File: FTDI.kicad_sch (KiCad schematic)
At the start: 14 parts, among them U6 FT2232HL-TRAY, Y2 12Mhz 20ppm

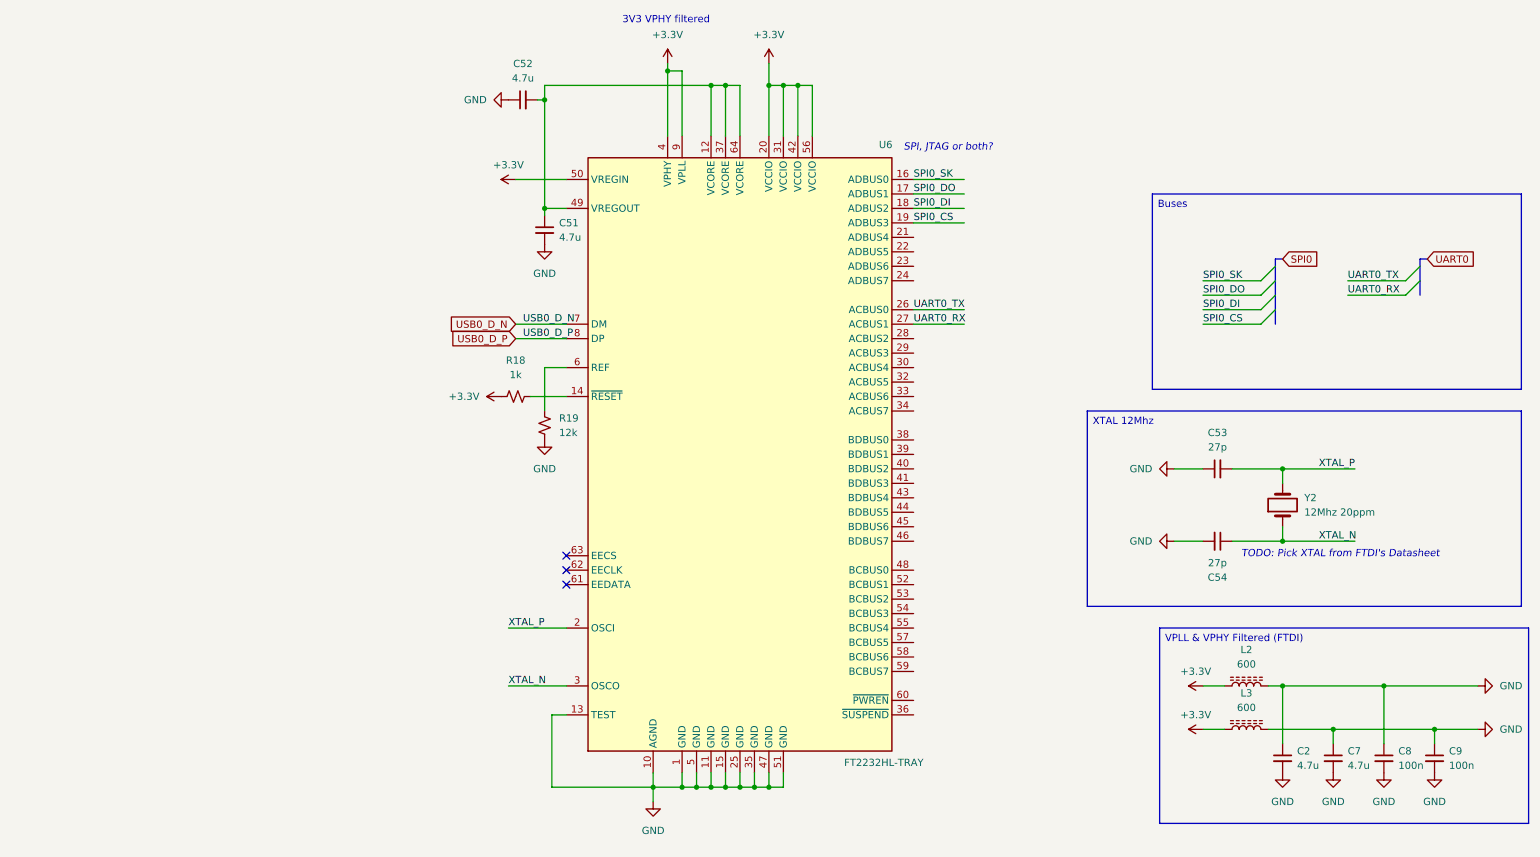
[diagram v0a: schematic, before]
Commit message: Alot of stuff
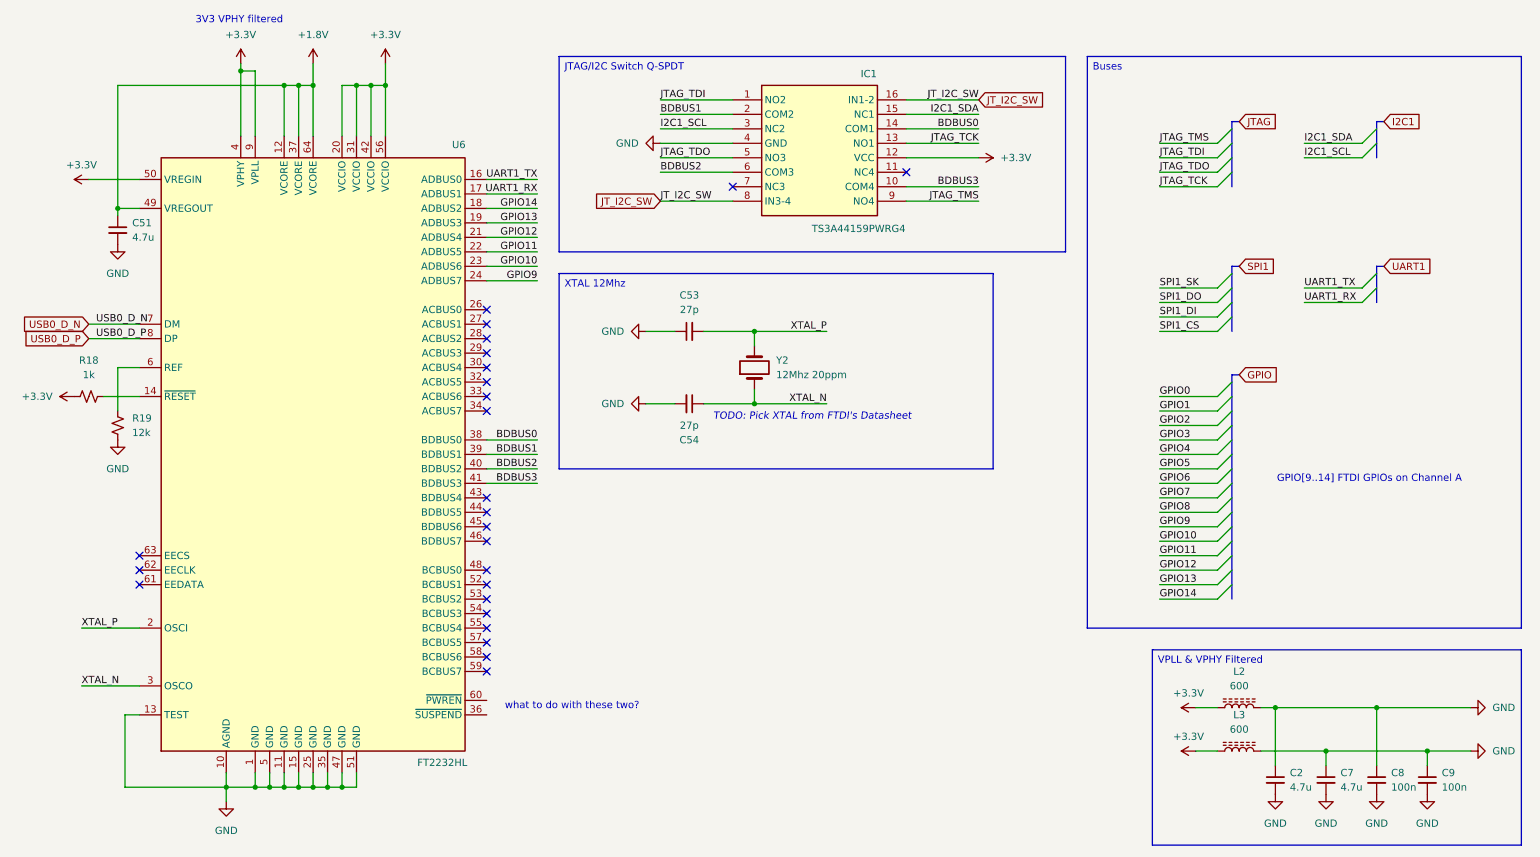
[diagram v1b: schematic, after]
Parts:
- removed C52: 4.7u, symbol Device:C_Small
- added IC1: TS3A44159PWRG4, SOP65P640X120-16N, symbol SamacSys_Parts:TS3A44159PWRG4
- U6: value FT2232HL-TRAY -> FT2232HL
- Y2: footprint (none) -> SamacSys_Parts:ABLS7
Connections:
- net +3.3V: now also IC1.12 (VCC)
- net GND: now also IC1.4 (GND)
- net +1.8V: now reaches C51.1, U6.12 (VCORE), U6.37 (VCORE), U6.49 (VREGOUT), U6.64 (VCORE)
- net GPIO12: now reaches U6.21 (ADBUS4)
- net GPIO11: now reaches U6.22 (ADBUS5)
- net GPIO10: now reaches U6.23 (ADBUS6)
- net GPIO9: now reaches U6.24 (ADBUS7)
- net BDBUS0: now reaches U6.38 (BDBUS0)
- net BDBUS0: now also IC1.14 (COM1)
- net BDBUS1: now reaches U6.39 (BDBUS1)
- net BDBUS1: now also IC1.2 (COM2)
- net BDBUS2: now reaches U6.40 (BDBUS2)
- net BDBUS2: now also IC1.6 (COM3)
- net BDBUS3: now reaches U6.41 (BDBUS3)
- net BDBUS3: now also IC1.10 (COM4)
- net SPI0_CS renamed GPIO13
- net SPI0_DI renamed GPIO14
- net SPI0_DO renamed UART1_RX
- net SPI0_SK renamed UART1_TX
- net UART0_RX: no longer names the net of U6.27 (ACBUS1)
- net UART0_TX: no longer names the net of U6.26 (ACBUS0)
- new net I2C1_SCL: IC1.3 (NC2)
- new net I2C1_SDA: IC1.15 (NC1)
- new net JTAG_TCK: IC1.13 (NO1)
- new net JTAG_TDI: IC1.1 (NO2)
- new net JTAG_TDO: IC1.5 (NO3)
- new net JTAG_TMS: IC1.9 (NO4)
- new net JT_I2C_SW: IC1.16 (IN1-2), IC1.8 (IN3-4)
- no-connect marks 3 -> 25
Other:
- note added: "GPIO[9..14] FTDI GPIOs on Channel A"
- note added: "what to do with these two?"
- note removed: "SPI, JTAG or both?"
- moved on the sheet: C2, C51, C53, C54, C7, C8, C9, L2, L3, R18, R19, U6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
